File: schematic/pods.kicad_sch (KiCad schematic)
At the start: 0 parts

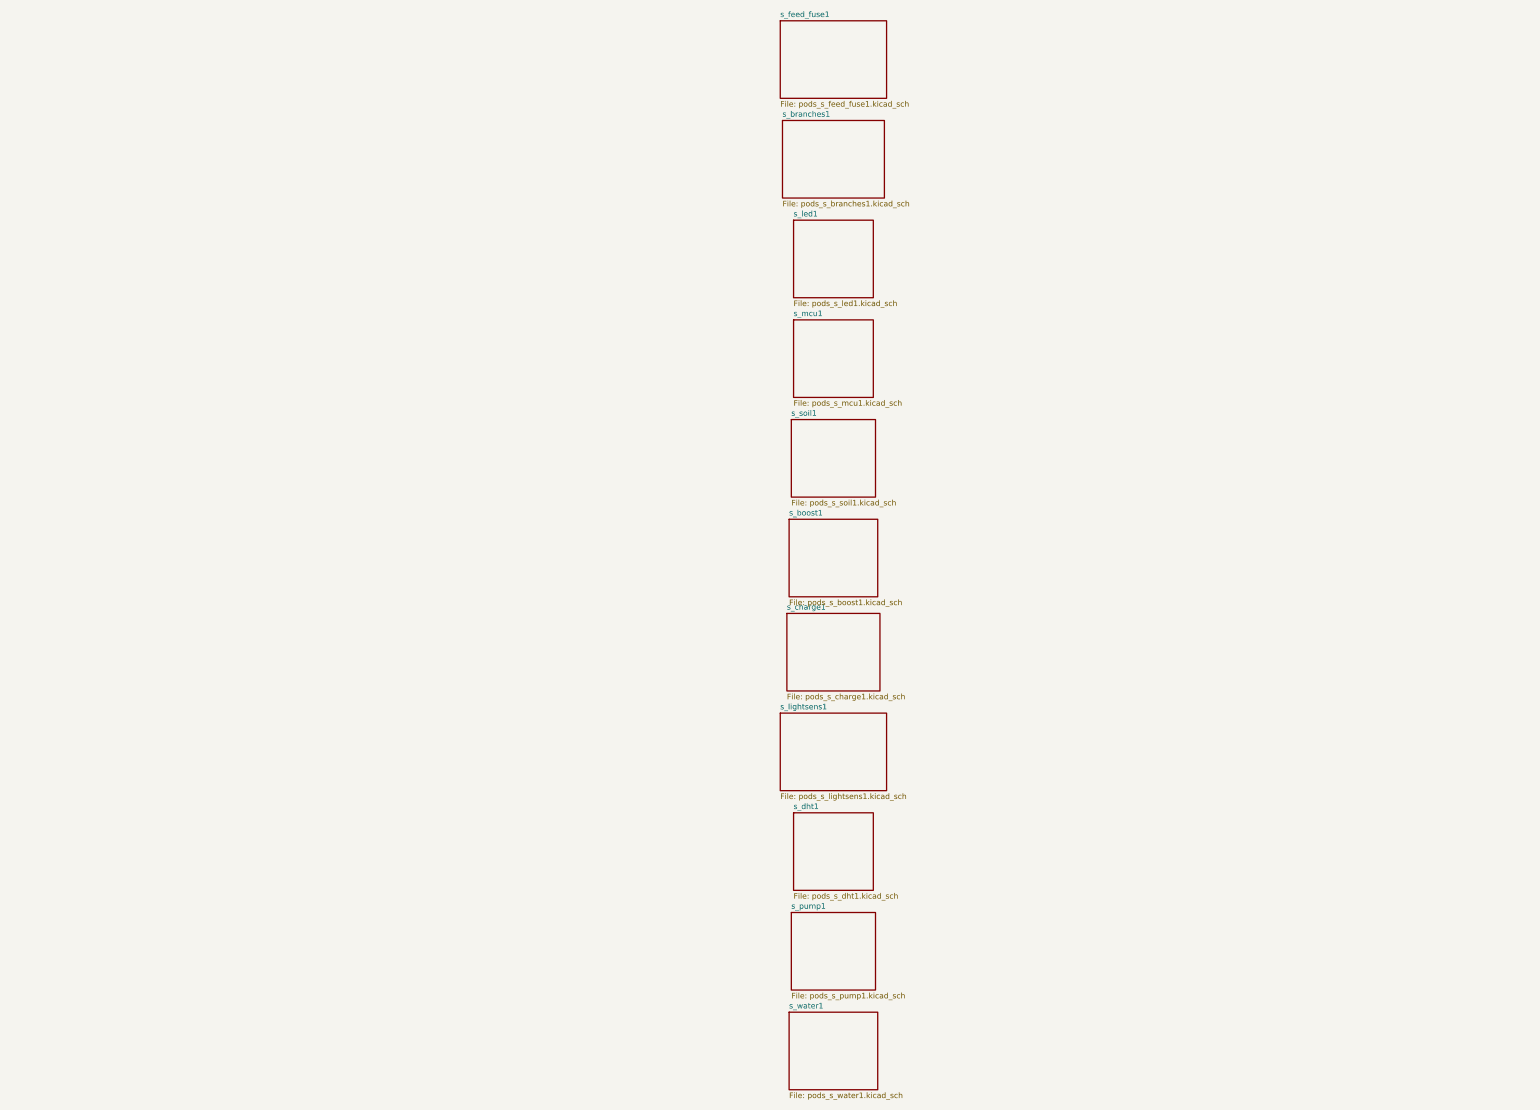
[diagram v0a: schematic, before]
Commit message: Regen SKiDL artifacts with flat draft (date/tag churn only, BOM stable at 41)
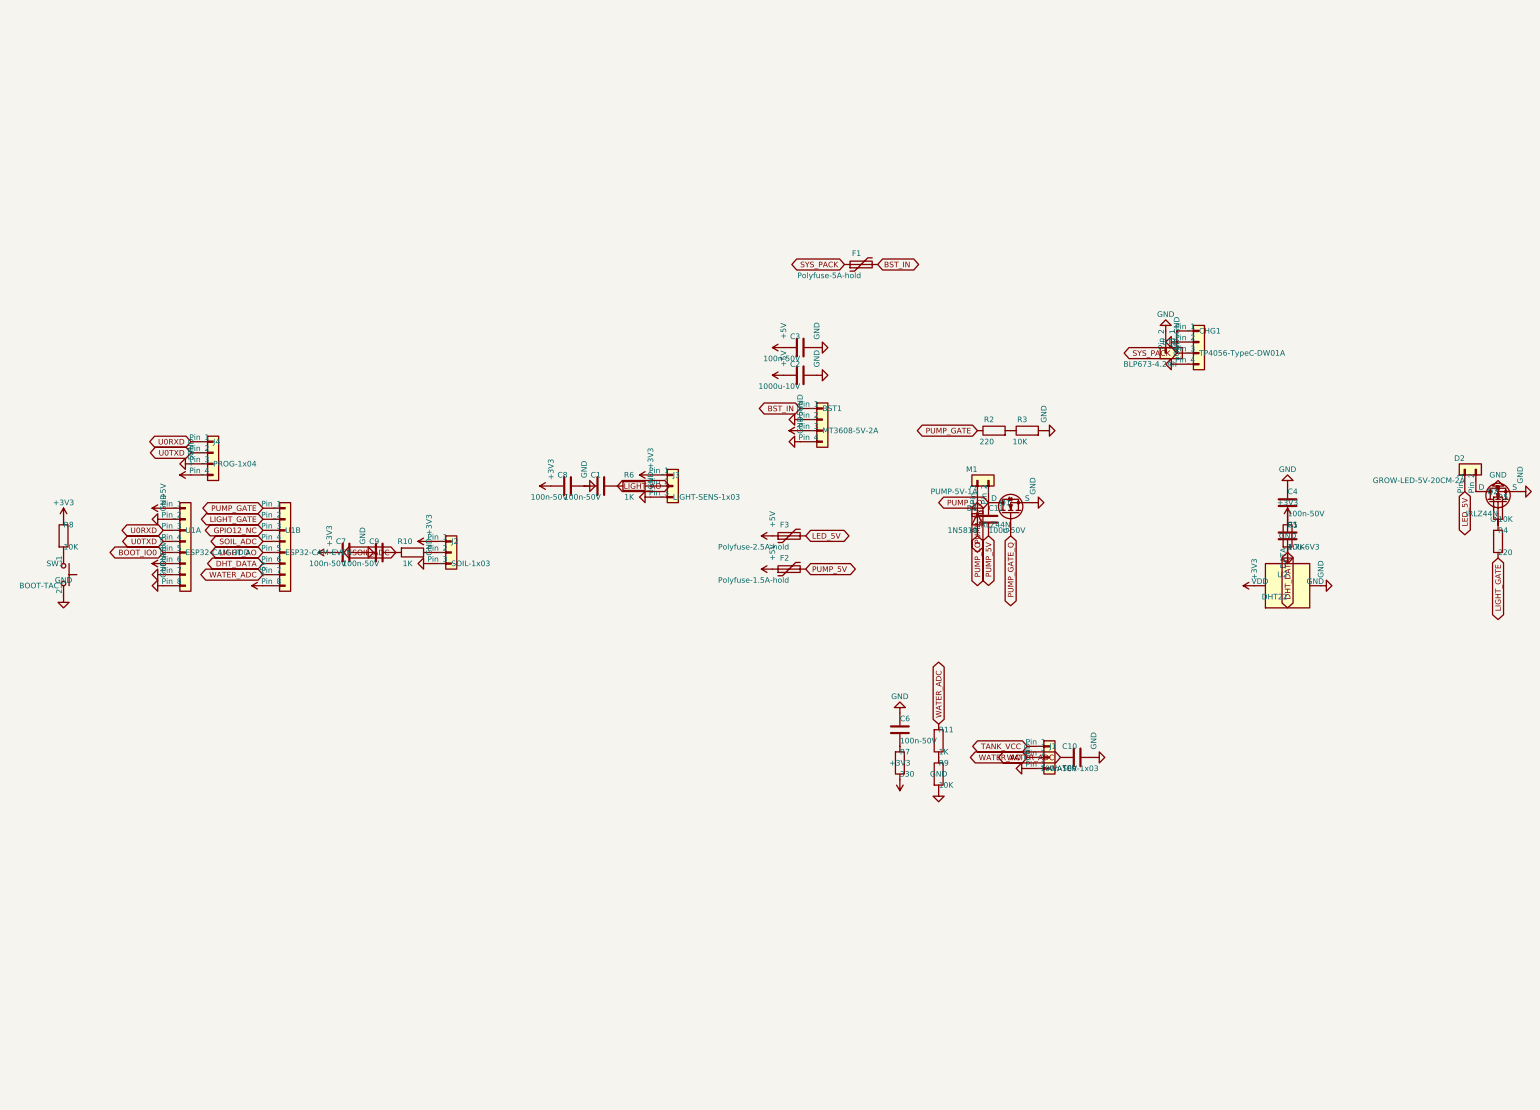
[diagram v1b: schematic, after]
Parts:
- added BST1: MT3608-5V-2A, Connector_PinHeader_2.54mm:PinHeader_1x04_P2.54mm_Vertical, symbol Connector_Generic:Conn_01x04
- added BT1: BLP673-4.2Ah, Connector_PinHeader_2.54mm:PinHeader_1x02_P2.54mm_Vertical, symbol Connector_Generic:Conn_01x02
- added C1, C10, C11, C3, C4, C6, C7, C8, C9: 100n-50V, Capacitor_SMD:C_0603_1608Metric, symbol Device:C
- added C2: 1000u-10V, Capacitor_THT:CP_Radial_D8.0mm_P3.50mm, symbol Device:C
- added C5: 10u-6V3, Capacitor_SMD:C_0603_1608Metric, symbol Device:C
- added CHG1: TP4056-TypeC-DW01A, Connector_PinHeader_2.54mm:PinHeader_1x04_P2.54mm_Vertical, symbol Connector_Generic:Conn_01x04
- added D1: 1N5819, Diode_THT:D_DO-41_SOD81_P7.62mm_Horizontal, symbol Diode:1N5819
- added D2: GROW-LED-5V-20CM-2A, Connector_PinHeader_2.54mm:PinHeader_1x02_P2.54mm_Vertical, symbol Connector_Generic:Conn_01x02
- added F1: Polyfuse-5A-hold, Fuse:Fuse_2920_7451Metric, symbol Device:Polyfuse
- added F2: Polyfuse-1.5A-hold, Fuse:Fuse_1812_4532Metric, symbol Device:Polyfuse
- added F3: Polyfuse-2.5A-hold, Fuse:Fuse_1812_4532Metric, symbol Device:Polyfuse
- added J1: WATER-1x03, Connector_PinHeader_2.54mm:PinHeader_1x03_P2.54mm_Vertical, symbol Connector_Generic:Conn_01x03
- added J2: SOIL-1x03, Connector_PinHeader_2.54mm:PinHeader_1x03_P2.54mm_Vertical, symbol Connector_Generic:Conn_01x03
- added J3: LIGHT-SENS-1x03, Connector_PinHeader_2.54mm:PinHeader_1x03_P2.54mm_Vertical, symbol Connector_Generic:Conn_01x03
- added J4: PROG-1x04, Connector_PinHeader_2.54mm:PinHeader_1x04_P2.54mm_Vertical, symbol Connector_Generic:Conn_01x04
- added M1: PUMP-5V-1A, Connector_PinHeader_2.54mm:PinHeader_1x02_P2.54mm_Vertical, symbol Connector_Generic:Conn_01x02
- added Q1, Q2: IRLZ44N, Package_TO_SOT_THT:TO-220-3_Vertical, symbol Transistor_FET:IRLZ44N
- added R1: 4.7K, Resistor_SMD:R_0603_1608Metric, symbol Device:R
- added R10, R11, R6: 1K, Resistor_SMD:R_0603_1608Metric, symbol Device:R
- added R2, R4: 220, Resistor_SMD:R_0603_1608Metric, symbol Device:R
- added R3, R5, R8, R9: 10K, Resistor_SMD:R_0603_1608Metric, symbol Device:R
- added R7: 330, Resistor_SMD:R_0603_1608Metric, symbol Device:R
- added SW1: BOOT-TACT, Button_Switch_THT:SW_PUSH-12mm, symbol Switch:SW_Push
- added U1A: ESP32-CAM-ODD, Connector_PinHeader_2.54mm:PinHeader_1x08_P2.54mm_Vertical, symbol Connector_Generic:Conn_01x08
- added U1B: ESP32-CAM-EVEN, Connector_PinHeader_2.54mm:PinHeader_1x08_P2.54mm_Vertical, symbol Connector_Generic:Conn_01x08
- added U2: DHT22, Connector_PinHeader_2.54mm:PinHeader_1x04_P2.54mm_Vertical, symbol Sensor:DHT11
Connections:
- new net: C6.1, R7.2
- new net: Q2.1 (G), R4.2, R5.1
- new net: R2.2, R3.1
- new net: J2.2 (Pin_2), R10.1
- new net: BT1.1 (Pin_1), CHG1.1 (Pin_1)
- new net: D2.2 (Pin_2), Q2.2 (D)
- new net: R8.2, SW1.1
- new net: R11.1, R9.1
- new net: J3.2 (Pin_2), R6.1
- new net +3V3: C4.1, C5.1, C7.1, C8.1, J2.1 (Pin_1), J3.1 (Pin_1), R1.1, R7.1, R8.1, U1A.6 (Pin_6), U2.1 (VDD)
- new net +5V: BST1.3 (Pin_3), C2.1, C3.1, F2.1, F3.1, J4.4 (Pin_4), U1A.1 (Pin_1), U1B.8 (Pin_8)
- new net BOOT_IO0: U1A.5 (Pin_5)
- new net BST_IN: BST1.1 (Pin_1), F1.2
- new net GND: BST1.2 (Pin_2), BST1.4 (Pin_4), BT1.2 (Pin_2), C1.2, C10.2, C2.2, C3.2, C4.2, C5.2, C6.2, C7.2, C8.2, C9.2, CHG1.2 (Pin_2), CHG1.4 (Pin_4), J1.3 (Pin_3), J2.3 (Pin_3), J3.3 (Pin_3), J4.3 (Pin_3), Q1.3 (S), Q2.3 (S), R1.2, R3.2, R5.2, R9.2, SW1.2, U1A.2 (Pin_2), U1A.7 (Pin_7), U1A.8 (Pin_8), U1B.6 (Pin_6), U2.2 (DATA), U2.4 (GND)
- new net GPIO12_NC: U1B.3 (Pin_3)
- new net LED_5V: D2.1 (Pin_1), F3.2
- new net LIGHT_AO: C1.1, R6.2, U1B.5 (Pin_5)
- new net LIGHT_GATE: R4.1, U1B.2 (Pin_2)
- new net PUMP_5V: C11.1, D1.1 (K), F2.2, M1.1 (Pin_1)
- new net PUMP_GATE: R2.1, U1B.1 (Pin_1)
- new net PUMP_GATE_Q: Q1.1 (G)
- new net PUMP_LO: C11.2, D1.2 (A), M1.2 (Pin_2), Q1.2 (D)
- new net SOIL_ADC: C9.1, R10.2, U1B.4 (Pin_4)
- new net SYS_PACK: CHG1.3 (Pin_3), F1.1
- new net TANK_VCC: J1.1 (Pin_1)
- new net U0RXD: J4.1 (Pin_1), U1A.3 (Pin_3)
- new net U0TXD: J4.2 (Pin_2), U1A.4 (Pin_4)
- new net WATER_ADC: C10.1, R11.2, U1B.7 (Pin_7)
- new net WATER_AO: J1.2 (Pin_2)
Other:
- removed sheet s_boost1
- removed sheet s_branches1
- removed sheet s_charge1
- removed sheet s_dht1
- removed sheet s_feed_fuse1
- removed sheet s_led1
- removed sheet s_lightsens1
- removed sheet s_mcu1
- removed sheet s_pump1
- removed sheet s_soil1
- removed sheet s_water1
